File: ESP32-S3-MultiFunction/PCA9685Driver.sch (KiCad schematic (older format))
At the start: 18 parts, among them P701 A7 A6 A5 A4 A3 A2 A1 A0 C, P702 B7 B6 B5 B4 B3 B2 B1 B0 C, T701 + 12V -, U701 PCA9685, U702 TBD62X83A, U703 TBD62X83A

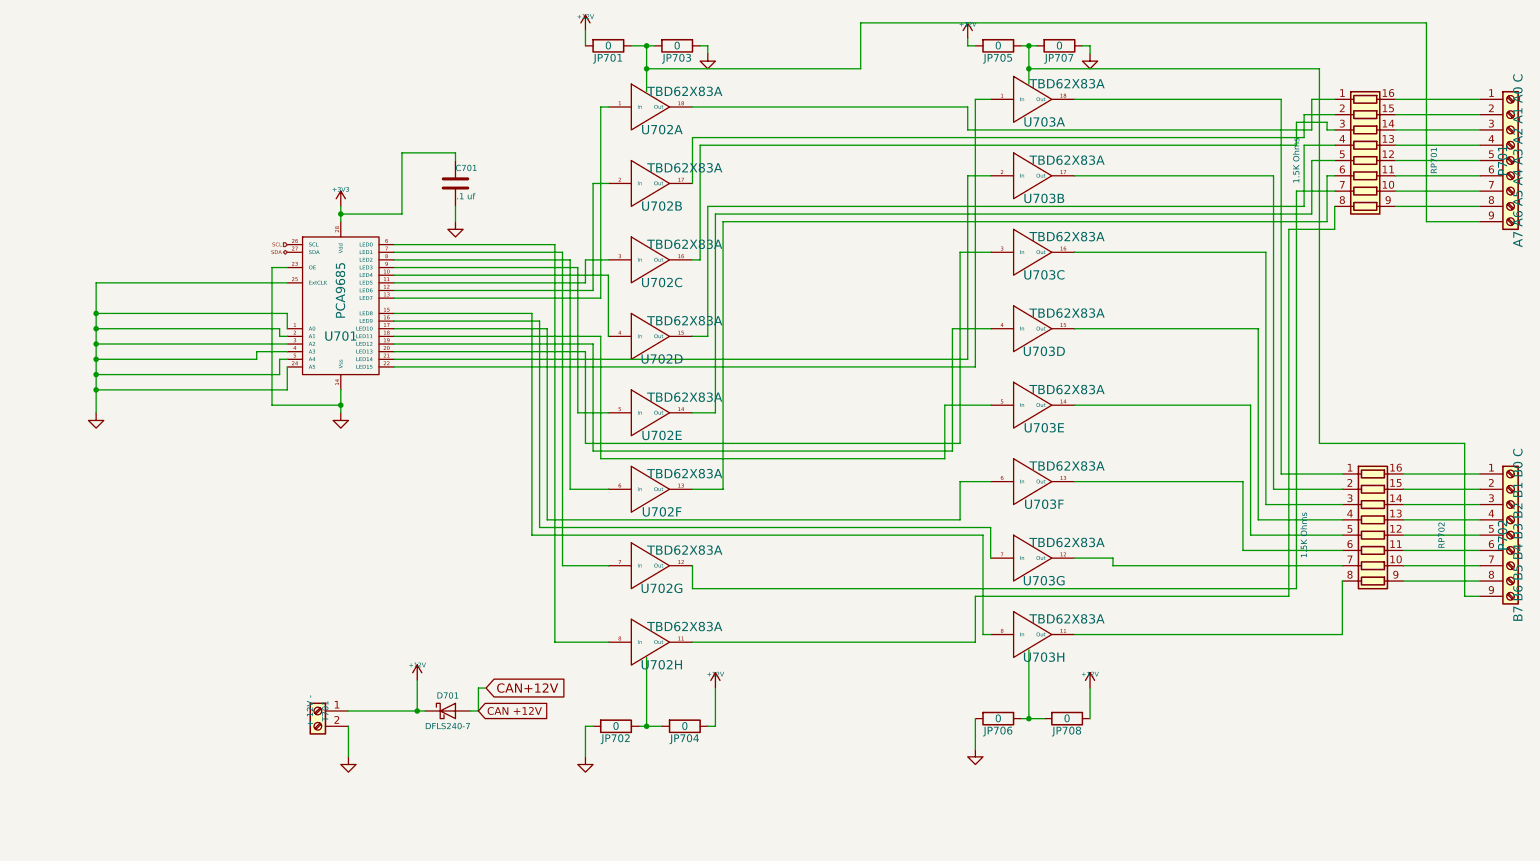
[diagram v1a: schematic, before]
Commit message: Create schematic PDF.
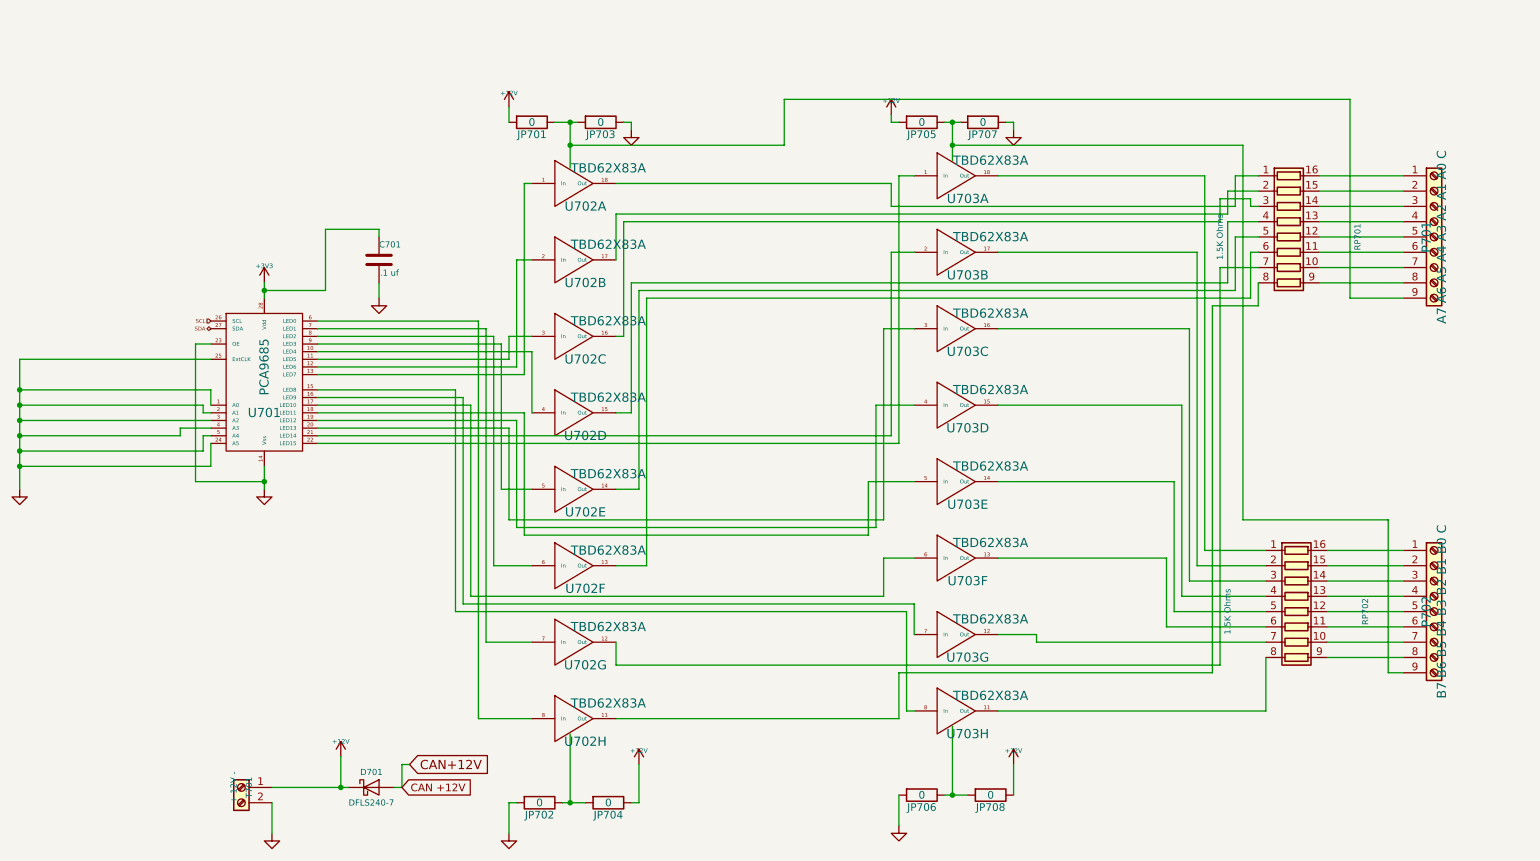
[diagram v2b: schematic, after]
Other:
- moved on the sheet: C701, D701, JP701, JP702, JP703, JP704, JP705, JP706, JP707, JP708, P701, P702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

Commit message: Fix minor part number and footprint error.
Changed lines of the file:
@@
 $EndComp
 Wire Wire Line
-	2300 3450 2300 3550
-Wire Wire Line
-	2300 3550 2300 3600
-Wire Wire Line
-	2300 2250 2300 2300
-Wire Wire Line
-	2300 2300 2300 2350
+	2300 3450 2300 3600
+Wire Wire Line
+	2300 2250 2300 2350
 Wire Wire Line
 	2700 2300 2700 1900
@@
 	3550 2950 2650 2950
 Wire Wire Line
-	4300 1200 4300 1350
-Wire Wire Line
-	4300 1350 4300 1500
-Wire Wire Line
-	6800 1200 6800 1350
-Wire Wire Line
-	6800 1350 6800 1450
+	4300 1200 4300 1500
+Wire Wire Line
+	6800 1200 6800 1450
 Wire Wire Line
 	6800 5150 6800 5600
@@
 	1900 3100 1900 3050
 Wire Wire Line
-	1900 3050 700  3050
+	700  3050 1900 3050
 Wire Wire Line
 	1950 3250 1900 3250
@@
 	700  3150 1950 3150
 Wire Wire Line
-	700  2750 700  2950
-Wire Wire Line
-	700  2950 700  3050
-Wire Wire Line
-	700  3050 700  3150
-Wire Wire Line
-	700  3150 700  3250
-Wire Wire Line
-	700  3250 700  3350
-Wire Wire Line
-	700  3350 700  3450
-Wire Wire Line
-	700  3450 700  3600
+	700  2750 700  3600
 Connection ~ 700  3050
 Connection ~ 700  3150
@@
 $EndComp
 Wire Wire Line
-	2350 5550 2800 5550
-Wire Wire Line
-	2800 5550 2850 5550
+	2350 5550 2850 5550
 $Comp
 L GND #PWR072
@@
 	3900 1100 3900 1200
 Wire Wire Line
-	4200 1200 4300 1200
-Wire Wire Line
-	4300 1200 4350 1200
+	4200 1200 4350 1200
 Connection ~ 4300 1200
 Wire Wire Line
@@
 $EndComp
 Wire Wire Line
-	4250 5650 4300 5650
-Wire Wire Line
-	4300 5650 4400 5650
+	4250 5650 4400 5650
 Connection ~ 4300 5650
 Wire Wire Line
@@
 	6400 1200 6450 1200
 Wire Wire Line
-	6750 1200 6800 1200
-Wire Wire Line
-	6800 1200 6850 1200
+	6750 1200 6850 1200
 Connection ~ 6800 1200
 Wire Wire Line
@@
 	7200 5400 7200 5600
 Wire Wire Line
-	6900 5600 6800 5600
-Wire Wire Line
-	6800 5600 6750 5600
+	6750 5600 6900 5600
 Connection ~ 6800 5600
 Wire Wire Line

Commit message: Add a terminal block to provide external stall motor power.
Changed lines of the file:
@@
 SDA
 $Comp
-L +3V3 #PWR059
+L +3V3 #PWR060
 U 1 1 62B01C3D
 P 2300 2250
-F 0 "#PWR059" H 2300 2210 30  0001 C CNN
+F 0 "#PWR060" H 2300 2210 30  0001 C CNN
 F 1 "+3V3" H 2300 2360 30  0000 C CNN
 F 2 "" H 2300 2250 60  0000 C CNN
@@
 $EndComp
 $Comp
-L GND #PWR060
+L GND #PWR061
 U 1 1 62B01C3E
 P 2300 3600
-F 0 "#PWR060" H 2300 3600 30  0001 C CNN
+F 0 "#PWR061" H 2300 3600 30  0001 C CNN
 F 1 "GND" H 2300 3530 30  0001 C CNN
 F 2 "" H 2300 3600 60  0000 C CNN
@@
 $EndComp
 $Comp
-L GND #PWR061
+L GND #PWR062
 U 1 1 62B01C40
 P 3050 2350
-F 0 "#PWR061" H 3050 2350 30  0001 C CNN
+F 0 "#PWR062" H 3050 2350 30  0001 C CNN
 F 1 "GND" H 3050 2280 30  0001 C CNN
 F 2 "" H 3050 2350 60  0000 C CNN
@@
 $EndComp
 $Comp
-L +12V #PWR062
+L +12V #PWR063
 U 1 1 62B01C55
 P 3900 1100
-F 0 "#PWR062" H 3900 1190 20  0001 C CNN
+F 0 "#PWR063" H 3900 1190 20  0001 C CNN
 F 1 "+12V" H 3900 1190 30  0000 C CNN
 F 2 "" H 3900 1100 60  0000 C CNN
@@
 $EndComp
 $Comp
-L +12V #PWR063
+L +12V #PWR064
 U 1 1 62B01C56
 P 6400 1150
-F 0 "#PWR063" H 6400 1240 20  0001 C CNN
+F 0 "#PWR064" H 6400 1240 20  0001 C CNN
 F 1 "+12V" H 6400 1240 30  0000 C CNN
 F 2 "" H 6400 1150 60  0000 C CNN
@@
 $EndComp
 $Comp
-L +12V #PWR064
+L +12V #PWR065
 U 1 1 62B01C57
 P 7200 5400
-F 0 "#PWR064" H 7200 5490 20  0001 C CNN
+F 0 "#PWR065" H 7200 5490 20  0001 C CNN
 F 1 "+12V" H 7200 5490 30  0000 C CNN
 F 2 "" H 7200 5400 60  0000 C CNN
@@
 $EndComp
 $Comp
-L +12V #PWR065
+L +12V #PWR066
 U 1 1 62B01C58
 P 4750 5400
-F 0 "#PWR065" H 4750 5490 20  0001 C CNN
+F 0 "#PWR066" H 4750 5490 20  0001 C CNN
 F 1 "+12V" H 4750 5490 30  0000 C CNN
 F 2 "" H 4750 5400 60  0000 C CNN
@@
 $EndComp
 $Comp
-L GND #PWR066
+L GND #PWR067
 U 1 1 62B01C59
 P 3900 5850
-F 0 "#PWR066" H 3900 5850 30  0001 C CNN
+F 0 "#PWR067" H 3900 5850 30  0001 C CNN
 F 1 "GND" H 3900 5780 30  0001 C CNN
 F 2 "" H 3900 5850 60  0000 C CNN
@@
 $EndComp
 $Comp
-L GND #PWR067
+L GND #PWR068
 U 1 1 62B01C5A
 P 6450 5800
-F 0 "#PWR067" H 6450 5800 30  0001 C CNN
+F 0 "#PWR068" H 6450 5800 30  0001 C CNN
 F 1 "GND" H 6450 5730 30  0001 C CNN
 F 2 "" H 6450 5800 60  0000 C CNN
@@
 $EndComp
 $Comp
-L GND #PWR068
+L GND #PWR069
 U 1 1 62B01C5B
 P 7200 1250
-F 0 "#PWR068" H 7200 1250 30  0001 C CNN
+F 0 "#PWR069" H 7200 1250 30  0001 C CNN
 F 1 "GND" H 7200 1180 30  0001 C CNN
 F 2 "" H 7200 1250 60  0000 C CNN
@@
 $EndComp
 $Comp
-L GND #PWR069
+L GND #PWR070
 U 1 1 62B01C5C
 P 4700 1250
-F 0 "#PWR069" H 4700 1250 30  0001 C CNN
+F 0 "#PWR070" H 4700 1250 30  0001 C CNN
 F 1 "GND" H 4700 1180 30  0001 C CNN
 F 2 "" H 4700 1250 60  0000 C CNN
@@
 $EndComp
 $Comp
-L GND #PWR070
+L GND #PWR071
 U 1 1 62B01C5D
 P 700 3600
-F 0 "#PWR070" H 700 3600 30  0001 C CNN
+F 0 "#PWR071" H 700 3600 30  0001 C CNN
 F 1 "GND" H 700 3530 30  0001 C CNN
 F 2 "" H 700 3600 60  0000 C CNN
@@
 	1900 3100 1900 3050
 Wire Wire Line
-	700  3050 1900 3050
+	1900 3050 700  3050
 Wire Wire Line
 	1950 3250 1900 3250
@@
 $EndComp
 $Comp
-L +12V #PWR071
+L +12V #PWR072
 U 1 1 62B01C5F
 P 2800 5350
-F 0 "#PWR071" H 2800 5300 20  0001 C CNN
+F 0 "#PWR072" H 2800 5300 20  0001 C CNN
 F 1 "+12V" H 2800 5450 30  0000 C CNN
 F 2 "" H 2800 5350 60  0000 C CNN
@@
 	2350 5550 2850 5550
 $Comp
-L GND #PWR072
+L GND #PWR073
 U 1 1 62B01C61
 P 2350 5850
-F 0 "#PWR072" H 2350 5850 30  0001 C CNN
+F 0 "#PWR073" H 2350 5850 30  0001 C CNN
 F 1 "GND" H 2350 5780 30  0001 C CNN
 F 2 "" H 2350 5850 60  0000 C CNN
